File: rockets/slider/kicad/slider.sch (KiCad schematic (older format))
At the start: 34 parts

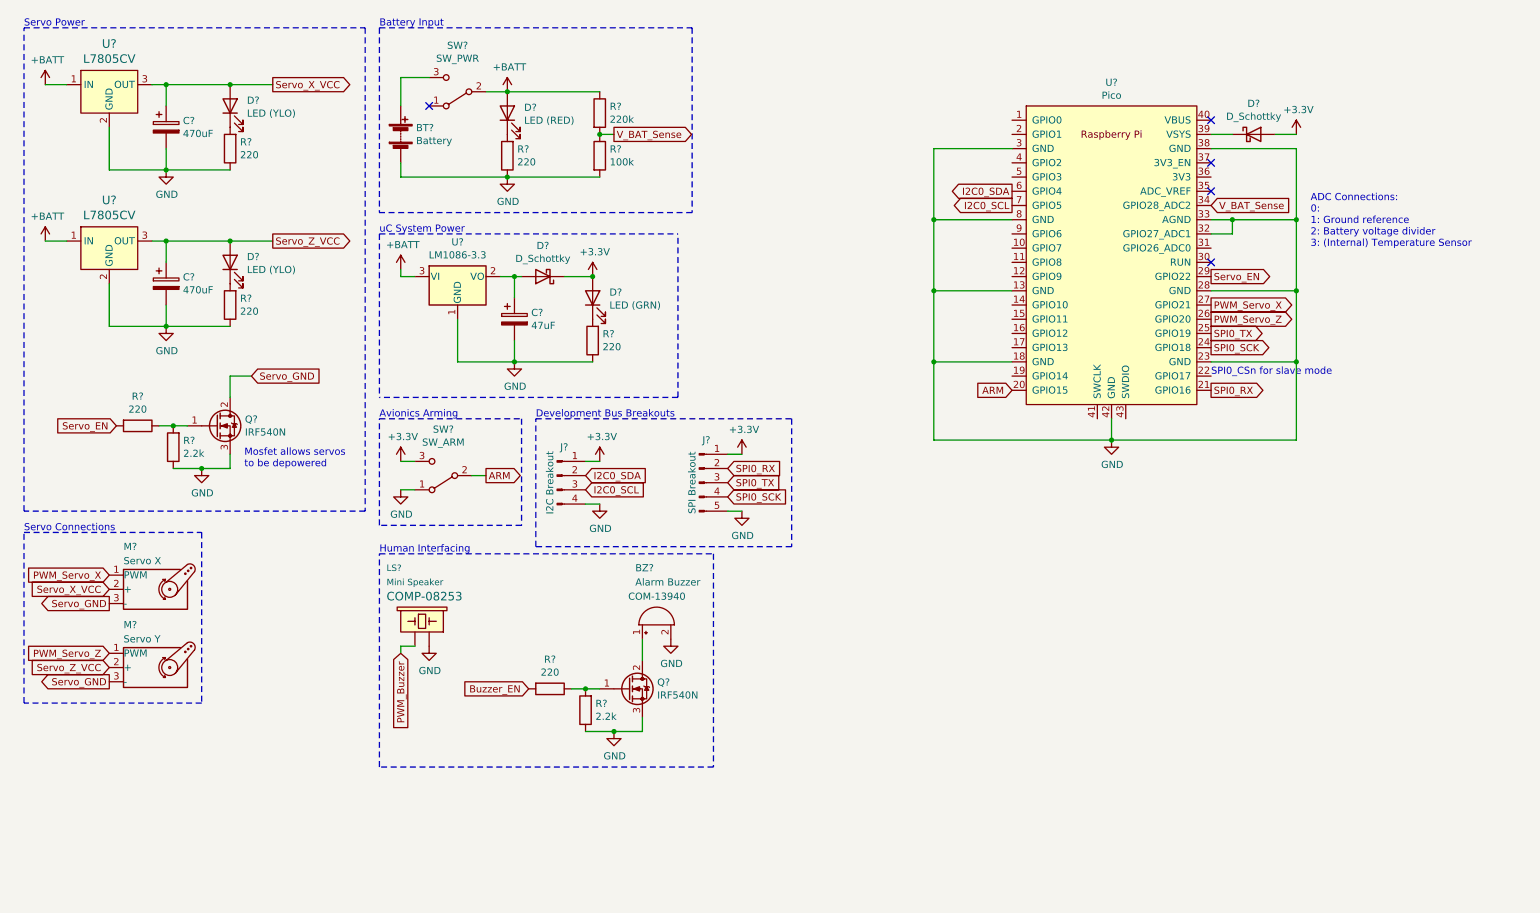
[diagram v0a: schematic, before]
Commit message: More shematic
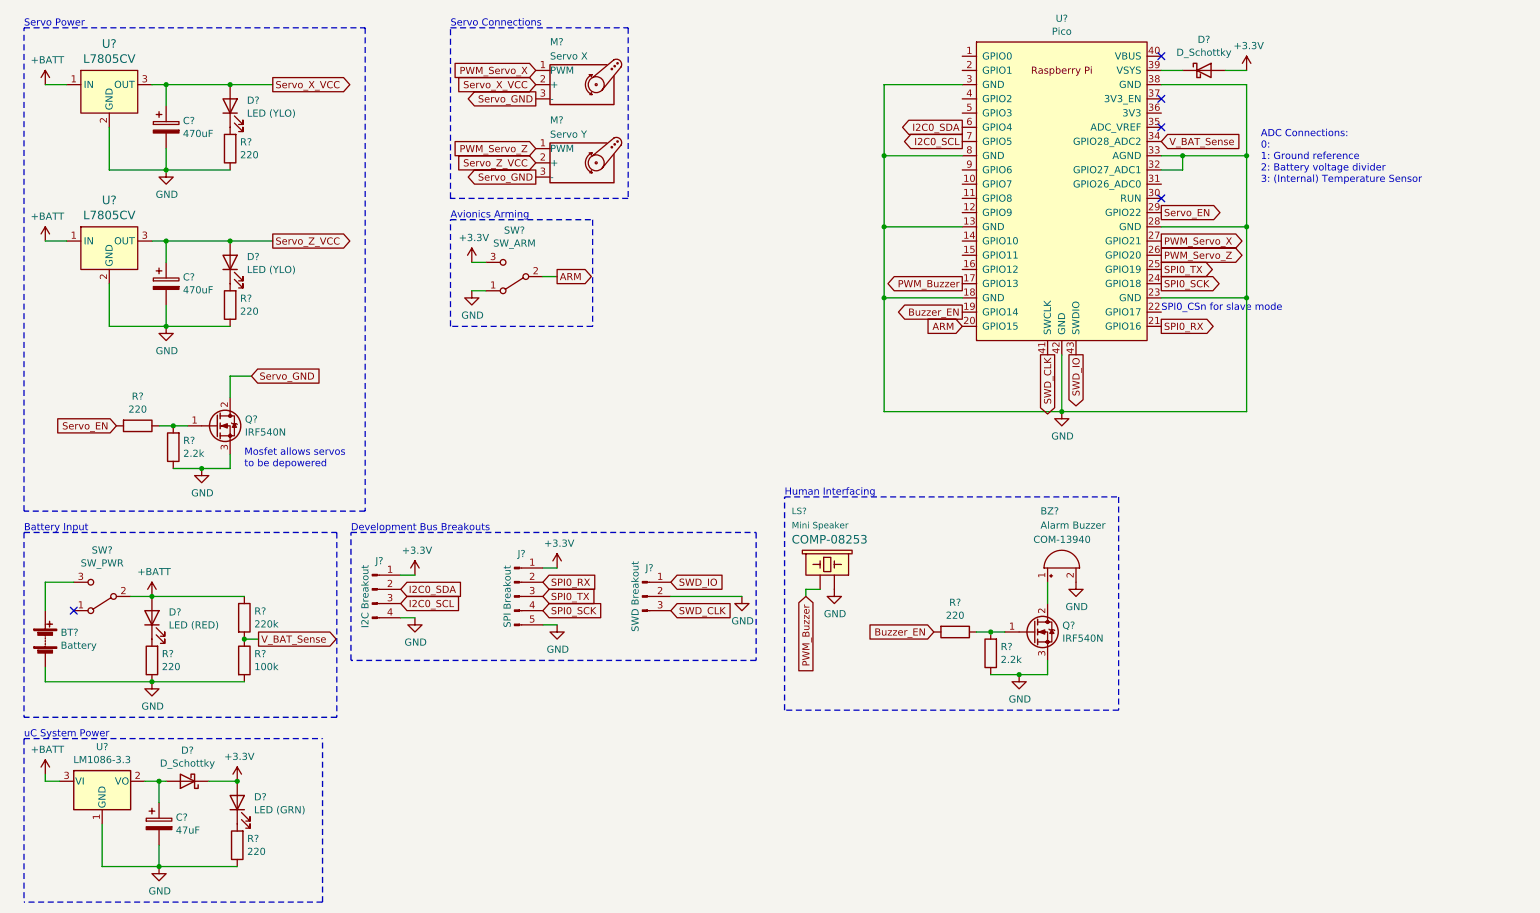
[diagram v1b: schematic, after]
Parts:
- added J?: SWD Breakout, symbol Connector:Conn_01x03_Male
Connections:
- net Buzzer_EN: now also U?.19 (GPIO14)
- net GND: now also J?.2 (Pin_2)
- net PWM_Buzzer: now also U?.17 (GPIO13)
- net SWD_CLK: now reaches U?.41 (SWCLK)
- net SWD_CLK: now also J?.3 (Pin_3)
- net SWD_IO: now reaches U?.43 (SWDIO)
- net SWD_IO: now also J?.1 (Pin_1)
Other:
- moved on the sheet: BT?, BZ?, C?, D?, J?, LS?, M?, Q?, R?, SW?, U?
